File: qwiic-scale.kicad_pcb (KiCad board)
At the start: 4 copper layers, 74.5 x 34.5 mm, 128 parts, among them J1 USB_B_Micro, J10 Conn_01x04, J11 Conn_01x02, J12 Conn_01x02, J13 BM03B-SRSS-TBLFSN, J2 Conn_02x05_Odd_Even, J3 SM04B-SRSS-TB(LF)(SN), J4 SM04B-SRSS-TB(LF)(SN), J5 Conn_01x04, J6 Conn_01x04, J7 Conn_01x04, J8 Conn_01x04, J9 Conn_01x02, Q7 DMN63D8LDW, Q8 DMN63D8LDW, Q9 DMN63D8LDW, SW1 SW_Push, SW2 SW_Push, U1 RP2040, U12 W25Q128JVS, U2 NAU7802SGI, U3 AP3012, U4 AMS1117-3.3, U5 NAU7802SGI, U7 ADM7170ACPZ-1.8-R7, Y1 XYDBPCNANF-12MHZ

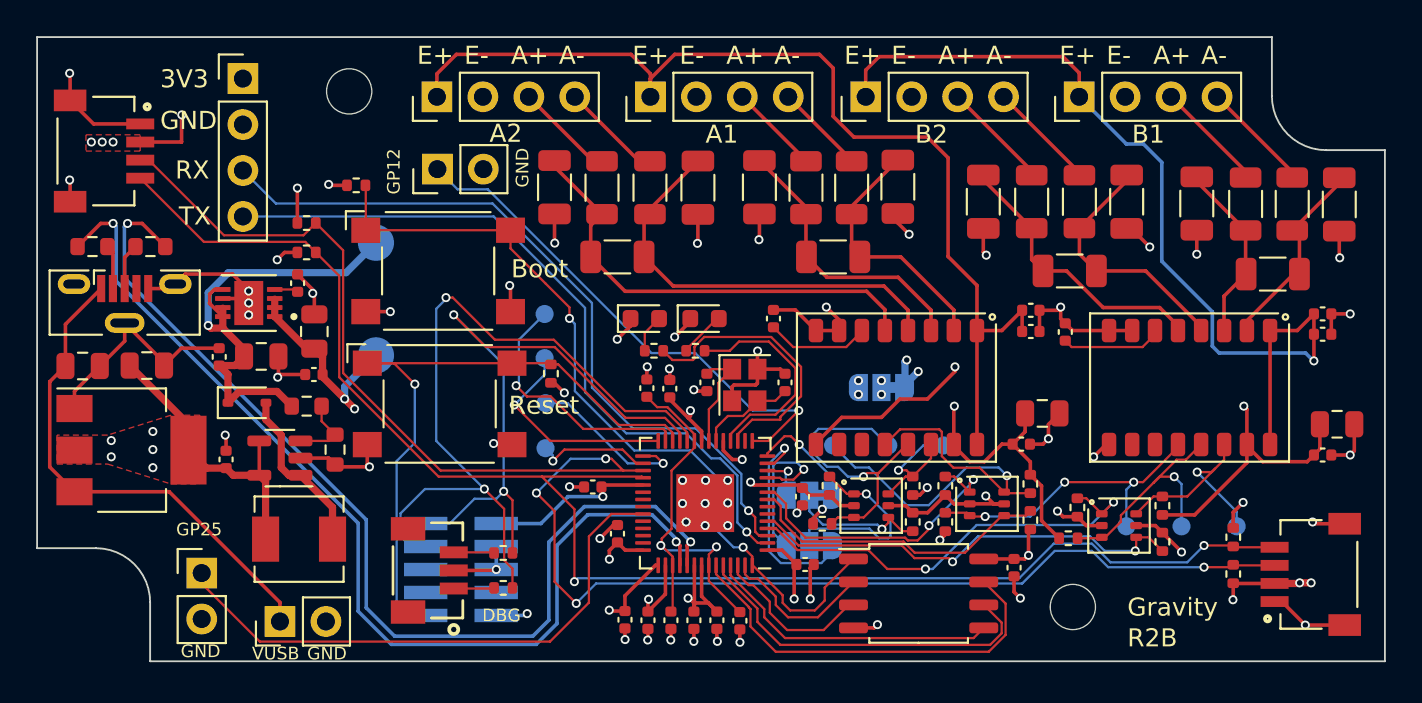
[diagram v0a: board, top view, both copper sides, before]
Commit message: WIP
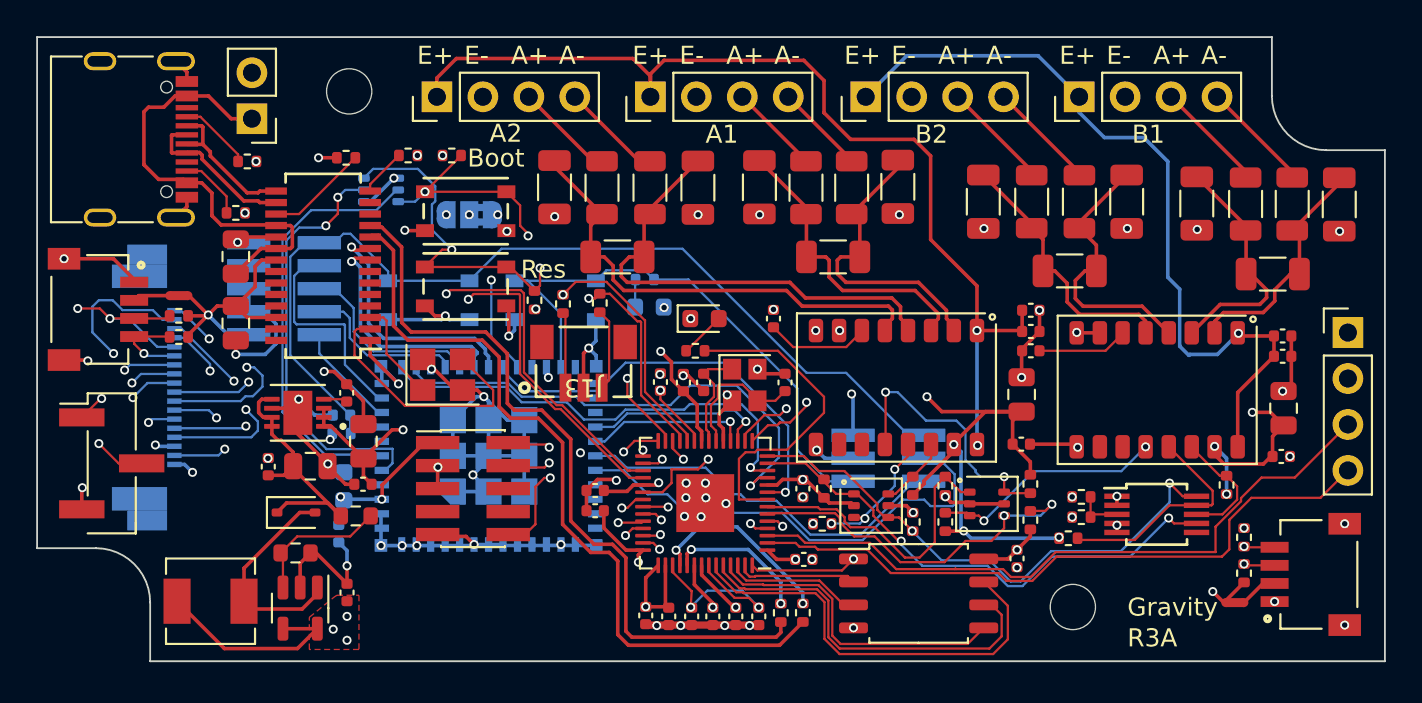
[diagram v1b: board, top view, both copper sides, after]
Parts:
- removed JP2, JP3: SolderJumper_3_Bridged12, Jumper:SolderJumper-3_P1.3mm_Bridged12_RoundedPad1.0x1.5mm
- removed Q9: DMN63D8LDW, PCM_Package_TO_SOT_SMD_AKL:SOT-363_SC-70-6
- removed TP1, TP2: TestPoint, TestPoint:TestPoint_Pad_D2.0mm
- removed TP10, TP11, TP12, TP7, TP8, TP9: TestPoint_Small, TestPoint:TestPoint_Pad_D1.0mm
- removed TP3, TP4, TP5, TP6: TestPoint, TestPoint:TestPoint_Pad_D1.0mm
- added C46: 1 uF, >6.3V, X5R, Capacitor_SMD:C_0402_1005Metric, B.Cu at (68.3, 104.4)
- added C47: 100 nF, >10V, X6S, Capacitor_SMD:C_0402_1005Metric, B.Cu at (68.2, 110.9)
- added C48: 22 uF, 6.3V, X5R, Capacitor_SMD:C_0603_1608Metric, B.Cu at (68.5, 108.3)
- added J14: USB_C_Receptacle_USB2.0, Connector_USB:USB_C_Receptacle_G-Switch_GT-USB-7010ASV, F.Cu at (56.1, 89.2)
- added J15: Conn_01x03, Connector_PinHeader_2.54mm:PinHeader_1x03_P2.54mm_Vertical_SMD_Pin1Left, F.Cu at (55.6, 107.1)
- added NT1: NetTie_2, NetTie:NetTie-2_SMD_Pad0.5mm, F.Cu at (59.3, 97.8)
- added NT2: NetTie_2, NetTie:NetTie-2_SMD_Pad0.5mm, F.Cu at (117.7, 114.8)
- added Q1: DMN63D8LDW, PCM_Package_TO_SOT_SMD_AKL:SOT-363_SC-70-6, B.Cu at (70.5, 91.9)
- added R35: 2K7 1%, Resistor_SMD:R_0402_1005Metric, F.Cu at (72.0, 90.0)
- added R36: 10K, Resistor_SMD:R_0402_1005Metric, F.Cu at (68.6, 90.2)
- added R37: 120R, Resistor_SMD:R_0402_1005Metric, B.Cu at (85.1, 96.9)
- added R38: 5K1, Resistor_SMD:R_0402_1005Metric, F.Cu at (62.5, 93.2)
- added R39: 5K1, Resistor_SMD:R_0402_1005Metric, F.Cu at (63.1, 90.4)
- added SW3: SW_Push, ul_PTS815-SJM-250-SMTR-LFS:SW4_PTS815 SJM 250 SMTR LFS_CNK, B.Cu at (80.1, 98.0)
- added SW4: SW_Push, ul_PTS815-SJM-250-SMTR-LFS:SW4_PTS815 SJM 250 SMTR LFS_CNK, B.Cu at (73.2, 98.0)
- added U6: ESP32-C6-MINI-1/U, PCM_Espressif:ESP32-C6-MINI-1, B.Cu at (76.5, 109.3)
- added U8: FE1.1s (Rev B), Package_SO:SSOP-28_3.9x9.9mm_P0.635mm, F.Cu at (67.3, 96.1)
- added Y3: 12MHz, Crystal:Crystal_SMD_3225-4Pin_3.2x2.5mm, F.Cu at (73.9, 102.2)
- D3: moved to B.Cu
- J1: value USB_B_Micro -> Molex_527461871; footprint Connector_USB:USB_Micro-B_Molex-105133-0001 -> CON_527461871_MOL:CON_527461871_MOL; moved to B.Cu
- J11: value Conn_01x02 -> Conn_02x05_Odd_Even; footprint Connector_PinHeader_2.54mm:PinHeader_1x02_P2.54mm_Vertical -> Connector_PinHeader_1.27mm:PinHeader_2x05_P1.27mm_Vertical_SMD; moved to B.Cu
- J12: value Conn_01x02 -> Conn_02x03_Odd_Even; footprint Connector_PinHeader_2.54mm:PinHeader_1x02_P2.54mm_Vertical -> Connector_PinHeader_1.27mm:PinHeader_2x03_P1.27mm_Vertical_SMD; moved to B.Cu
- J2: moved to F.Cu
- JP1: footprint Jumper:SolderJumper-3_P1.3mm_Bridged12_RoundedPad1.0x1.5mm -> Jumper:SolderJumper-3_P1.3mm_Bridged2Bar12_RoundedPad1.0x1.5mm_NumberLabels
- R26: value 10K -> 976K
- R28: value 10K -> 182K
- R32: value 120R -> 10K; moved to B.Cu
- R5, R6: footprint Resistor_SMD:R_0603_1608Metric -> Resistor_SMD:R_0402_1005Metric
- SW1, SW2: footprint Button_Switch_SMD:SW_SPST_Omron_B3FS-100xP -> ul_PTS815-SJM-250-SMTR-LFS:SW4_PTS815 SJM 250 SMTR LFS_CNK
- U4: value AMS1117-3.3 -> LTC4316CMS_PBF; footprint Package_TO_SOT_SMD:SOT-223-3_TabPin2 -> Package_SO:MSOP-10_3x3mm_P0.5mm
- moved J10 62.7 mm to (124.0, 99.8)
- moved U4 56.8 mm to (113.4, 109.9)
- moved R6 44.2 mm to (93.8, 115.3), turned to 90 degrees
- moved R5 40.3 mm to (92.6, 115.3), turned to 90 degrees
- moved J12 29.6 mm to (98.6, 106.8), turned to 180 degrees
- moved J9 27.8 mm to (63.4, 88.0), turned to 180 degrees
- moved JP1 24.7 mm to (75.4, 93.3)
- moved R32 17.9 mm to (68.3, 105.4), turned to 0 degrees
- moved J11 16.4 mm to (65.2, 97.4)
- moved R33 16.0 mm to (80.6, 98.2), turned to -90 degrees
- moved R34 14.8 mm to (82.6, 98.2), turned to 90 degrees
- moved J13 14.4 mm to (81.7, 101.5), turned to 180 degrees
- moved C36 10.4 mm to (62.5, 95.6), turned to 90 degrees
- moved C38 9.94 mm to (68.6, 114.2)
- moved J3 8.76 mm to (56.9, 98.6)
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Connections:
- C10 pad 2: QWIIC_VIN -> +3V3
- C11 pad 2: QWIIC_VIN -> +3V3
- C12 pad 1: QWIIC_VIN -> +3V3
- C13 pad 1: QWIIC_VIN -> +3V3
- C14 pad 1: QWIIC_VIN -> +3V3
- C15 pad 2: QWIIC_VIN -> +3V3
- C20 pad 1: +5VA -> AVCC
- C35 pad 2: +5VA -> AVCC
- C36 pad 1: RP2040_USB_VBUS -> USB_VBUS
- C38 pad 1: QWIIC_VIN -> +3V3
- C39 pad 1: QWIIC_VIN -> +3V3
- C6 pad 2: QWIIC_VIN -> +3V3
- C7 pad 2: QWIIC_VIN -> +3V3
- C8 pad 2: QWIIC_VIN -> +3V3
- C9 pad 2: QWIIC_VIN -> +3V3
- J1 pad 1: RP2040_USB_VBUS -> +3V3
- J1 pad 2: /RP2040_USB_POST_R_DN -> EYESPI_BL
- J1 pad 3: /RP2040_USB_POST_R_DP -> GND
- J1 pad 4: unconnected-(J1-ID-Pad4) -> EYESPI_SCK
- J1 pad 5: GND -> EYESPI_MOSI
- J1 pad 6: GND -> EYESPI_MISO
- J10 pad 1: QWIIC_VIN -> +3V3
- J11 pad 1: USER_BUTTON_1 -> +3V3
- J11 pad 2: GND -> ESP32_TMS
- J12 pad 1: USER_BUTTON_2 -> ESP32_EN
- J12 pad 2: GND -> +3V3
- J2 pad 1: QWIIC_VIN -> +3V3
- J3 pad 2: QWIIC_VIN -> QWIIC_VIN1
- J4 pad 2: QWIIC_VIN -> QWIIC_VIN2
- J9 pad 1: RP2040_USB_VBUS -> USB_VBUS
- JP1 pad 1: +5VA -> GND
- JP1 pad 2: AVCC -> ESP32_JTAG_SELECT
- JP1 pad 3: QWIIC_VIN -> +3V3
- L1 pad 1: QWIIC_VIN -> +3V3
- Q7 pad 2: QWIIC_VIN -> +3V3
- Q7 pad 5: QWIIC_VIN -> +3V3
- Q8 pad 2: QWIIC_VIN -> +3V3
- Q8 pad 5: QWIIC_VIN -> +3V3
- R1 pad 2: QWIIC_VIN -> +3V3
- R10 pad 2: QWIIC_VIN -> +3V3
- R2 pad 1: Net-(U1-GPIO15) -> Net-(U1-GPIO6)
- R20 pad 1: QWIIC_VIN -> +3V3
- R22 pad 1: QWIIC_VIN -> +3V3
- R24 pad 1: QWIIC_VIN -> +3V3
- R26 pad 1: QWIIC_VIN -> +3V3
- R26 pad 2: NAU7802_2_SDIO_3V3 -> Net-(U4-XORL)
- R28 pad 1: QWIIC_VIN -> Net-(U4-XORL)
- R28 pad 2: NAU7802_2_SCLK_3V3 -> GND
- R3 pad 2: QWIIC_VIN -> +3V3
- R30 pad 1: QWIIC_VIN -> +3V3
- R32 pad 1: Net-(U1-GPIO14) -> +3V3
- R32 pad 2: Net-(D3-A) -> ESP32_EN
- R7 pad 1: QWIIC_VIN -> +3V3
- R8 pad 2: QWIIC_VIN -> +3V3
- R9 pad 1: QWIIC_VIN -> +3V3
- U1 pad 1: QWIIC_VIN -> +3V3
- U1 pad 10: QWIIC_VIN -> +3V3
- U1 pad 11: NAU7802_1_SDIO_3V3_ALT_B -> RP2040_ESP32_TX
- U1 pad 12: NAU7802_1_SCLK_3V3_ALT_B -> RP2040_ESP32_RX
- U1 pad 13: NAU7802_1_SDIO_3V3_ALT_A -> NAU7802_1_SDIO_3V3
- U1 pad 14: NAU7802_1_SCLK_3V3_ALT_A -> NAU7802_1_SCLK_3V3
- U1 pad 15: USER_BUTTON_2 -> USER_2
- U1 pad 16: unconnected-(U1-GPIO13-Pad16) -> USER_1
- U1 pad 17: Net-(U1-GPIO14) -> RP2040_ESP32_GP1
- U1 pad 18: Net-(U1-GPIO15) -> RP2040_ESP32_GP2
- U1 pad 22: QWIIC_VIN -> +3V3
- U1 pad 27: Net-(U1-GPIO16) -> EYESPI_MISO
- U1 pad 28: Net-(U1-GPIO17) -> EYESPI_DISP_CS
- U1 pad 29: Net-(U1-GPIO18) -> EYESPI_SCK
- U1 pad 30: Net-(U1-GPIO19) -> EYESPI_MOSI
- U1 pad 33: QWIIC_VIN -> +3V3
- U1 pad 34: unconnected-(U1-GPIO22-Pad34) -> EYESPI_RES
- U1 pad 35: unconnected-(U1-GPIO23-Pad35) -> EYESPI_DC
- U1 pad 36: unconnected-(U1-GPIO24-Pad36) -> EYESPI_BUSY_TE
- U1 pad 37: USER_BUTTON_1 -> EYESPI_INT
- U1 pad 38: unconnected-(U1-GPIO26_ADC0-Pad38) -> EYESPI_BL
- U1 pad 39: unconnected-(U1-GPIO27_ADC1-Pad39) -> EYESPI_TS_CS
- U1 pad 4: NAU7802_2_SDIO_3V3 -> EYESPI_GP1
- U1 pad 40: unconnected-(U1-GPIO28_ADC2-Pad40) -> EYESPI_MEM_CS
- U1 pad 41: unconnected-(U1-GPIO29_ADC3-Pad41) -> EYESPI_SD_CS
- U1 pad 42: QWIIC_VIN -> +3V3
- U1 pad 43: QWIIC_VIN -> +3V3
- U1 pad 44: QWIIC_VIN -> +3V3
- U1 pad 48: QWIIC_VIN -> +3V3
- U1 pad 49: QWIIC_VIN -> +3V3
- U1 pad 5: NAU7802_2_SCLK_3V3 -> EYESPI_GP2
- U1 pad 6: unconnected-(U1-GPIO4-Pad6) -> NAU7802_2_DRDY_3V3
- U1 pad 7: unconnected-(U1-GPIO5-Pad7) -> NAU7802_1_DRDY_3V3
- U1 pad 8: NAU7802_2_DRDY_3V3 -> Net-(U1-GPIO6)
- U1 pad 9: NAU7802_1_DRDY_3V3 -> RP2040_SERIAL_BOOT
- U12 pad 8: QWIIC_VIN -> +3V3
- U3 pad 4: QWIIC_VIN -> +3V3
- U3 pad 5: QWIIC_VIN -> +3V3
- U4 pad 2: QWIIC_VIN -> GND
- U4 pad 3: RP2040_USB_VBUS -> Net-(U4-XORL)
- U7 pad 1: +5VA -> AVCC
- U7 pad 2: +5VA -> AVCC
- U7 pad 3: +5VA -> AVCC
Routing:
- net QWIIC_VIN: track 91.9 -> 0.00 mm, vias 31 -> 0
- net +3V3: track 0.00 -> 85.4 mm, vias 0 -> 29
- net USER_2: track 0.00 -> 59.6 mm, vias 0 -> 2
- net EYESPI_GP1: track 0.00 -> 56.2 mm, vias 0 -> 3
- net ESP32_EN: track 0.00 -> 54.9 mm
- net USER_1: track 0.00 -> 51.0 mm, vias 0 -> 2
- net +5VA: track 49.9 -> 0.00 mm, vias 4 -> 0
- net RP2040_USB_PRE_R_DP: track 55.7 -> 7.85 mm
- net EYESPI_GP2: track 0.00 -> 46.3 mm, vias 0 -> 2
- net RP2040_USB_PRE_R_DN: track 55.5 -> 10.6 mm
- net EYESPI_RES: track 0.00 -> 42.2 mm, vias 0 -> 2
- net /RP2040_USB_POST_R_DN: track 2.45 -> 43.0 mm
- net /RP2040_USB_POST_R_DP: track 2.57 -> 41.9 mm
- net EYESPI_SD_CS: track 0.00 -> 38.8 mm, vias 0 -> 2
- net AVCC: track 69.3 -> 107.5 mm, vias 7 -> 9
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- added copper zone on F.Cu, net +3V3
- added copper zone on In1.Cu, net +3V3
- added copper zone on In2.Cu, net GND
- removed copper zone on In1.Cu, net GND
- removed copper zone on F.Cu, net QWIIC_VIN
- removed copper zone on In2.Cu, net QWIIC_VIN
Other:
- copper layers 4 -> 6
- board text added: "EN"
- board text added: "GP0"
- board text added: "R3A"
- board text removed: "3V3"
- board text removed: "5VA"
- board text removed: "6V2"
- board text removed: "DBG"
- board text removed: "GND"
- board text removed: "GP12"
- board text removed: "GP16"
- board text removed: "GP17"
- board text removed: "GP18"
- board text removed: "GP19"
- board text removed: "GP25"
- board text removed: "R2B"
- board text removed: "RX"
- board text removed: "Reset"
- board text removed: "SWCLK"
- board text removed: "SWD"
- board text removed: "TX"
- board text removed: "VUSB"
